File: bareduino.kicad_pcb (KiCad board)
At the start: 2 copper layers, 21.6 x 39.4 mm, 18 parts, among them J1 AVR-ISP-6, J2 Conn_01x15_Male, J3 Conn_01x15_Male, U1 AP2204K-5.0, U2 ATmega328P-AU, U3 AP2204K-3.3, Y1 Crystal

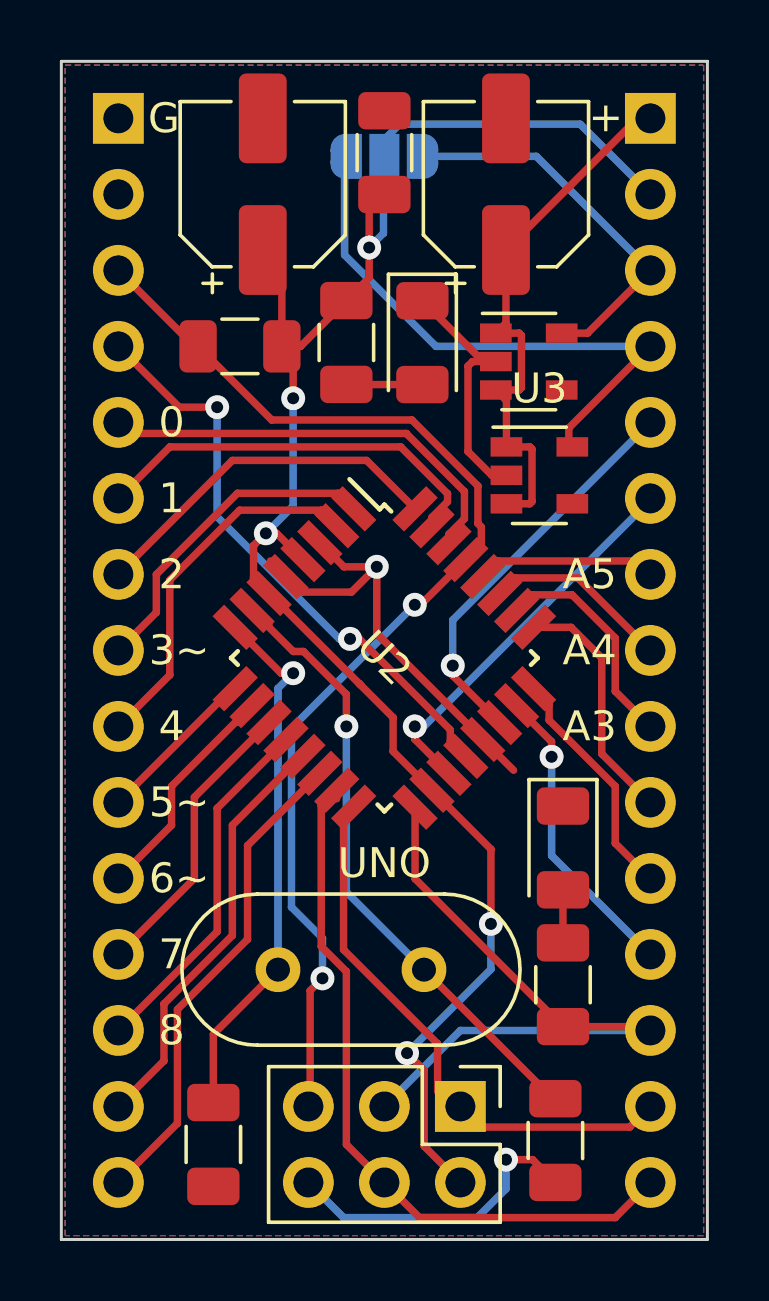
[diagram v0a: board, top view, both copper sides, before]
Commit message: revision B
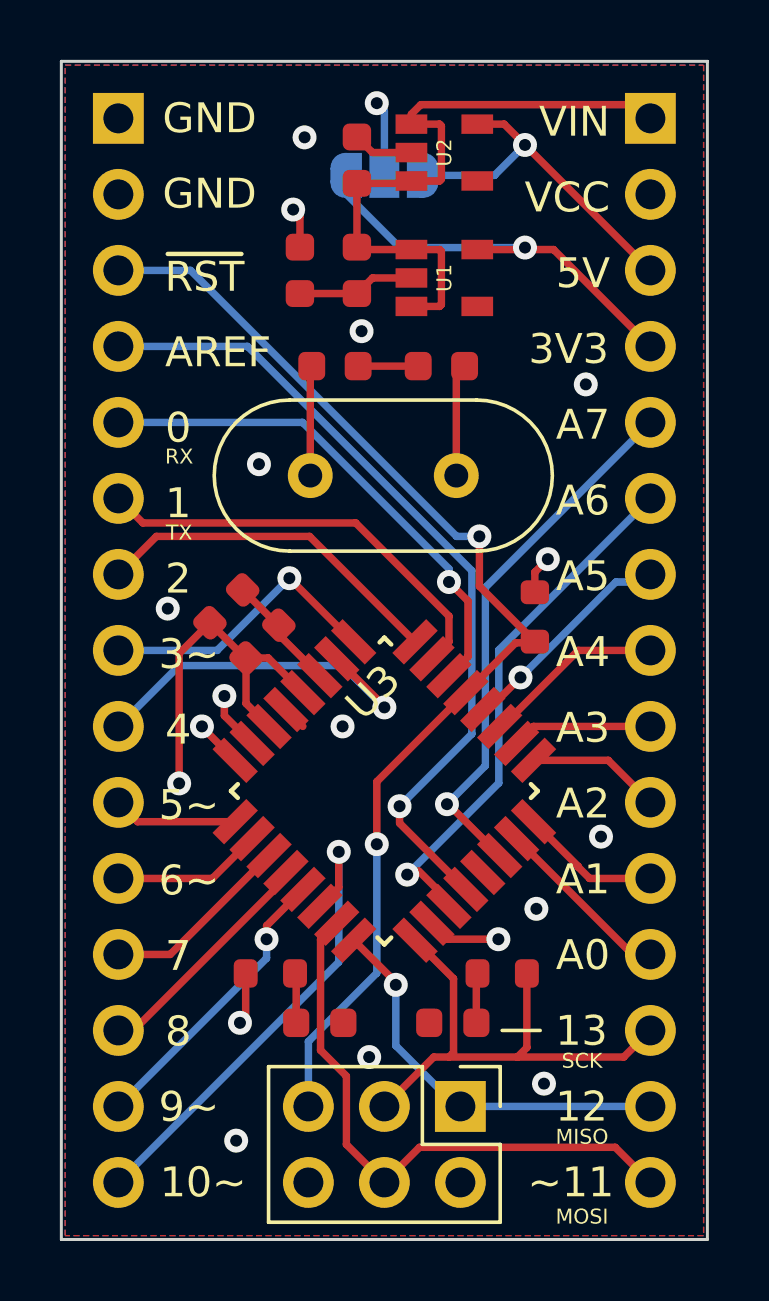
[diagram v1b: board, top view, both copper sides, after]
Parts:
- removed the C2 at (48.0, 54.3)
- added C1: 1u, kicad-official/Capacitor_SMD.pretty:C_0603_1608Metric, F.Cu at (51.2, 57.1)
- added C4: 100n, kicad-official/Capacitor_SMD.pretty:C_0603_1608Metric, F.Cu at (48.0, 69.6)
- added C5: 1u, kicad-official/Capacitor_SMD.pretty:C_0603_1608Metric, F.Cu at (46.8, 68.4)
- C2: renamed from C1; value 100u -> 1u; footprint Capacitor_SMD:CP_Elec_5x5.8 -> kicad-official/Capacitor_SMD.pretty:C_0603_1608Metric
- C3: value .1u -> 2.2u; footprint Capacitor_SMD:C_1206_3216Metric -> kicad-official/Capacitor_SMD.pretty:C_0603_1608Metric
- C6: renamed from C4; value .1u -> 22p; footprint Capacitor_SMD:C_1206_3216Metric -> kicad-official/Capacitor_SMD.pretty:C_0603_1608Metric
- C7: renamed from C5; value .1u -> 22p; footprint Capacitor_SMD:C_1206_3216Metric -> kicad-official/Capacitor_SMD.pretty:C_0603_1608Metric
- D1, D2: footprint LED_SMD:LED_1206_3216Metric -> kicad-official/LED_SMD.pretty:LED_0603_1608Metric
- R1, R2, R3: footprint Resistor_SMD:R_1206_3216Metric -> kicad-official/Resistor_SMD.pretty:R_0603_1608Metric
- moved C6 26.3 mm to (50.4, 60.4), turned to 0 degrees
- moved C7 26.2 mm to (54.0, 60.4), turned to 180 degrees
- moved D2 23.0 mm to (49.9, 82.3), turned to 180 degrees
- moved R2 21.2 mm to (48.3, 80.6), turned to 0 degrees
- moved Y1 16.5 mm to (49.6, 64.0)
- moved R3 13.4 mm to (57.1, 68.7), turned to -90 degrees
- moved U2 7.53 mm to (54.1, 53.2)
- moved U1 7.32 mm to (54.1, 57.4)
- moved D1 6.91 mm to (54.4, 82.3), turned to 0 degrees
- moved C2 5.05 mm to (51.2, 53.5)
- moved C3 4.84 mm to (49.2, 57.1), turned to -90 degrees
- moved U3 4.45 mm to (52.1, 74.5)
- moved R1 2.07 mm to (56.0, 80.6), turned to 180 degrees
- moved JP1 0.63 mm to (52.1, 54.0)
- renumbered U3 to U1, U1 to U2, U2 to U3
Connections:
- net /~RESET renamed /~{RESET}
- U1 pad 4: Net-(U3-Pad4) -> unconnected-(U1-Pad4)
- U2 pad 4: Net-(U1-Pad4) -> unconnected-(U2-Pad4)
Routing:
- net VCC: track 60.2 -> 95.0 mm, vias 5 -> 6
- net GND: track 34.9 -> 12.5 mm, vias 2 -> 11
- net /AREF: track 20.0 -> 27.5 mm, vias 2 -> 1
- net /MISO: track 19.3 -> 13.5 mm, vias 0 -> 1
- net Net-(C7-Pad1): track 21.7 -> 16.2 mm
- net +3V3: track 19.3 -> 13.9 mm, vias 0 -> 1
- net /SCK: track 22.3 -> 17.4 mm
- net /P8: track 12.0 -> 7.20 mm
- net /MOSI: track 24.3 -> 19.6 mm
- net /A0: track 10.2 -> 5.47 mm, vias 1 -> 0
- net /A7: track 13.4 -> 18.0 mm
- net /P9: track 14.3 -> 9.81 mm, vias 0 -> 1
- net /A6: track 13.1 -> 17.4 mm
- net /A2: track 8.20 -> 4.49 mm
- net /P7: track 9.84 -> 6.40 mm
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- added copper zone on In1.Cu, net GND
- added copper zone on In2.Cu, net GND
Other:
- copper layers 2 -> 4
- net class Default removed
- board text added: "10~"
- board text added: "11~"
- board text added: "12"
- board text added: "13"
- board text added: "3~"
- board text added: "5~"
- board text added: "6~"
- board text added: "9~"
- board text added: "MISO"
- board text added: "MOSI"
- board text added: "RX"
- board text added: "Rev B. OCT 24"
- board text added: "SCK"
- board text added: "TX"
- board text added: "~10"
- board text added: "~11"
- board text added: "~3"
- board text added: "~5"
- board text added: "~6"
- board text added: "~9"
- board text added: "~{RST}"
- board text removed: "+"
- board text removed: "11 O"
- board text removed: "12 I"
- board text removed: "13 C"
- board text removed: "3~~"
- board text removed: "5~~"
- board text removed: "6~~"
- board text removed: "G"
- board text removed: "RABID.AUDIO AUG 2021"
- board text removed: "UNO"
- board text removed: "~RST"
- board text removed: "~~10"
- board text removed: "~~3"
- board text removed: "~~5"
- board text removed: "~~6"
- board text removed: "~~9"
